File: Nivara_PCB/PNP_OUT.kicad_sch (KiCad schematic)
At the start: 12 parts, among them Q3 IRLML0040, Q4 IRLML0040, U10 LTV-357T, U11 LTV-357T

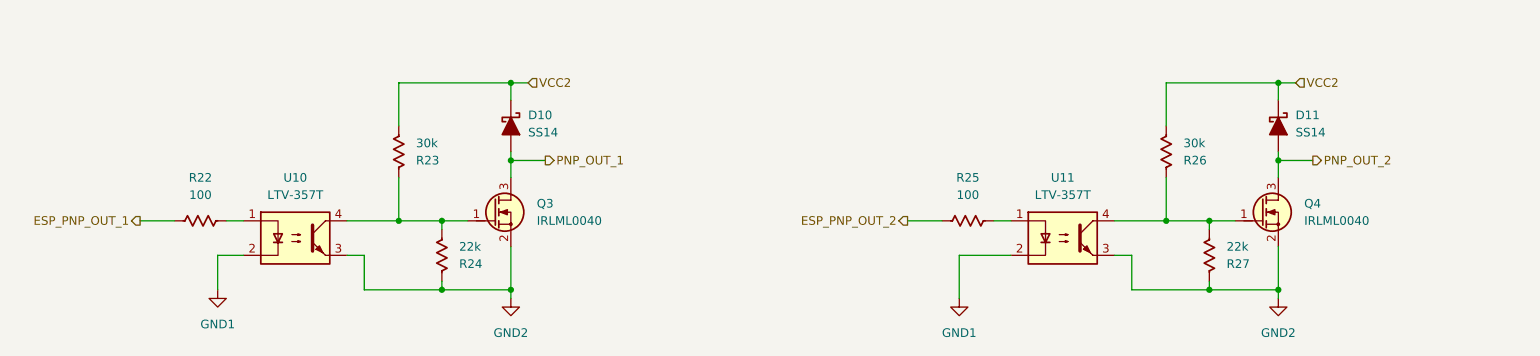
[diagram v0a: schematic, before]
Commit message: New changes to the Nivara PCB schematic files.
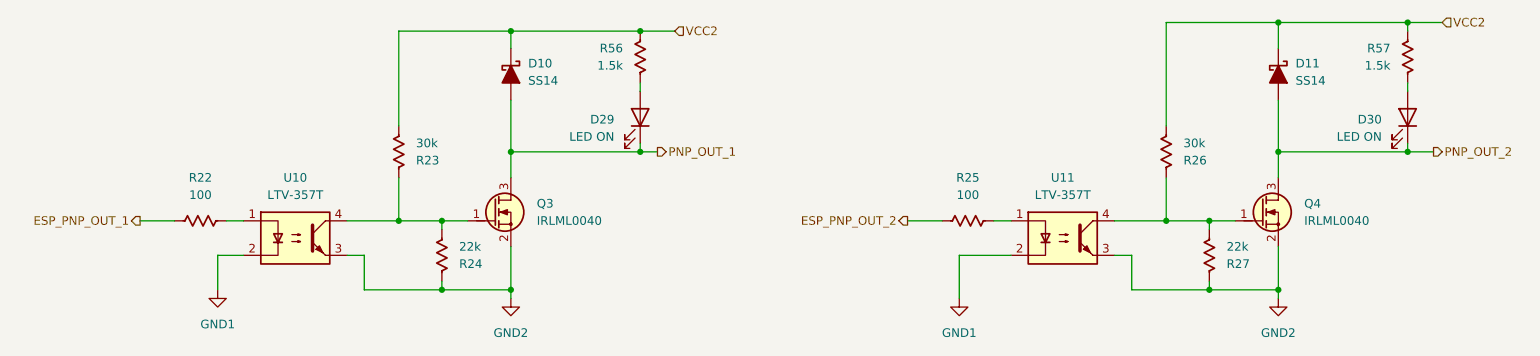
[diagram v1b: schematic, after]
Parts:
- added D29, D30: LED ON, LED_SMD:LED_0603_1608Metric, symbol Device:LED
- added R56, R57: 1.5k, PCM_Resistor_SMD_AKL:R_0603_1608Metric, symbol PCM_Resistor_US_AKL:R_0603
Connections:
- net PNP_OUT_1: now also D29.1 (K)
- net PNP_OUT_2: now also D30.1 (K)
- net VCC2: now also R56.1, R57.1
- new net: D29.2 (A), R56.2
- new net: D30.2 (A), R57.2
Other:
- moved on the sheet: D10
